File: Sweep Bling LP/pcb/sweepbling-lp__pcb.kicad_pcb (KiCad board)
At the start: 2 copper layers, 216.9 x 86.9 mm, 93 parts, among them J1 Conn_01x05, J1_r1 Conn_01x05, SW1 SW_Push, SW10 SW_Push, SW10_r1 SW_Push, SW11 SW_Push, SW11_r1 SW_Push, SW12 SW_Push, SW12_r1 SW_Push, SW13 SW_Push, SW13_r1 SW_Push, SW14 SW_Push, SW14_r1 SW_Push, SW15 SW_Push, SW15_r1 SW_Push, SW16 SW_Push, SW16_r1 SW_Push, SW17 SW_Push, SW17_r1 SW_Push, SW1_r1 SW_Push, SW2 SW_Push, SW2_r1 SW_Push, SW3 SW_Push, SW3_r1 SW_Push, SW4 SW_Push, SW4_r1 SW_Push, SW5 SW_Push, SW5_r1 SW_Push, SW6 SW_Push, SW6_r1 SW_Push, SW7 SW_Push, SW7_r1 SW_Push, SW8 SW_Push, SW8_r1 SW_Push, SW9 SW_Push, SW9_r1 SW_Push, U1 ProMicro-kbd, U2 ProMicro-kbd

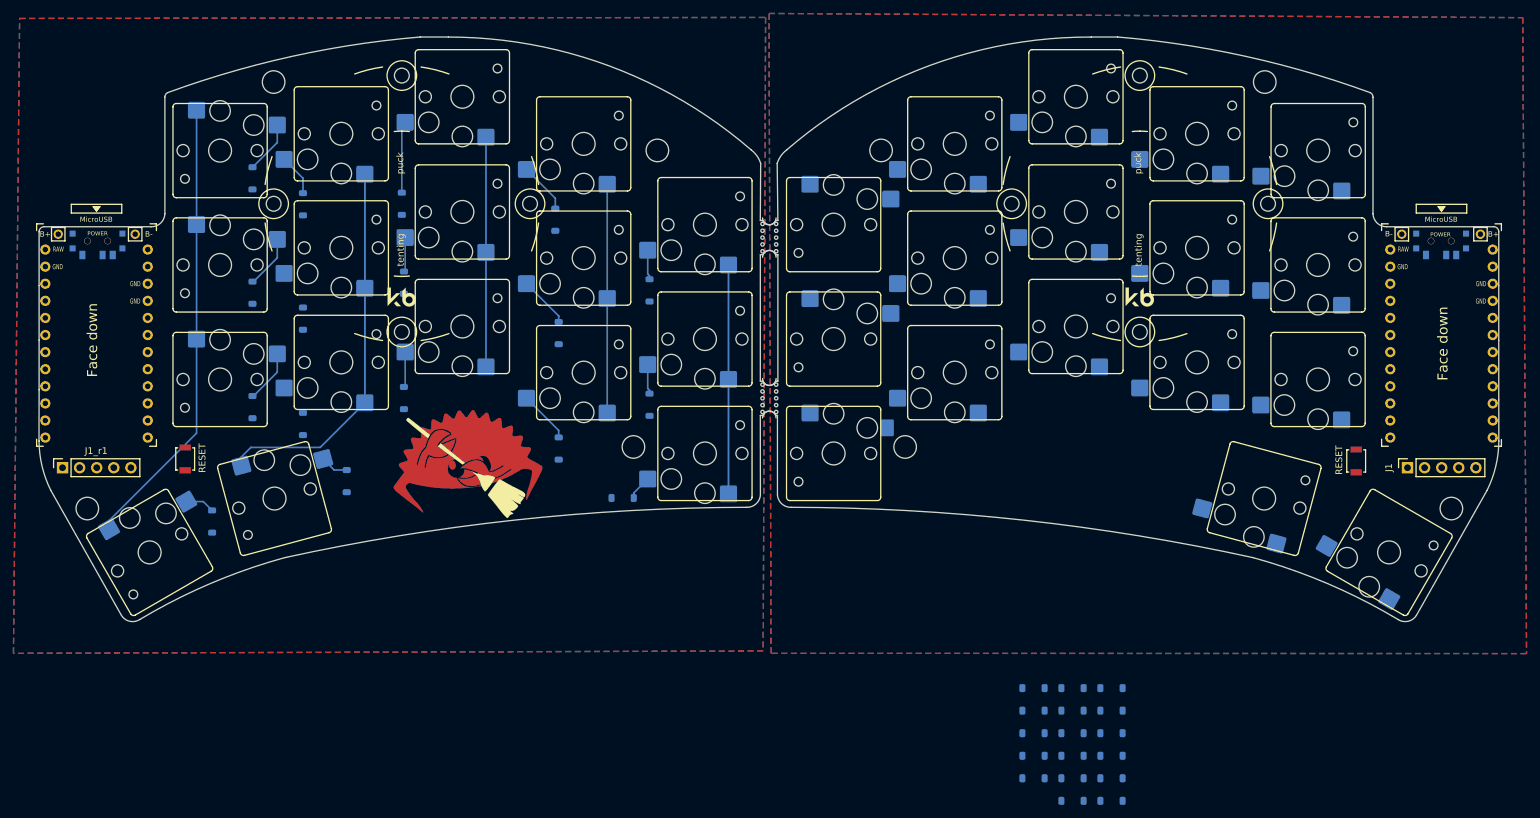
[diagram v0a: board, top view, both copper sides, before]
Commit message: traces addition
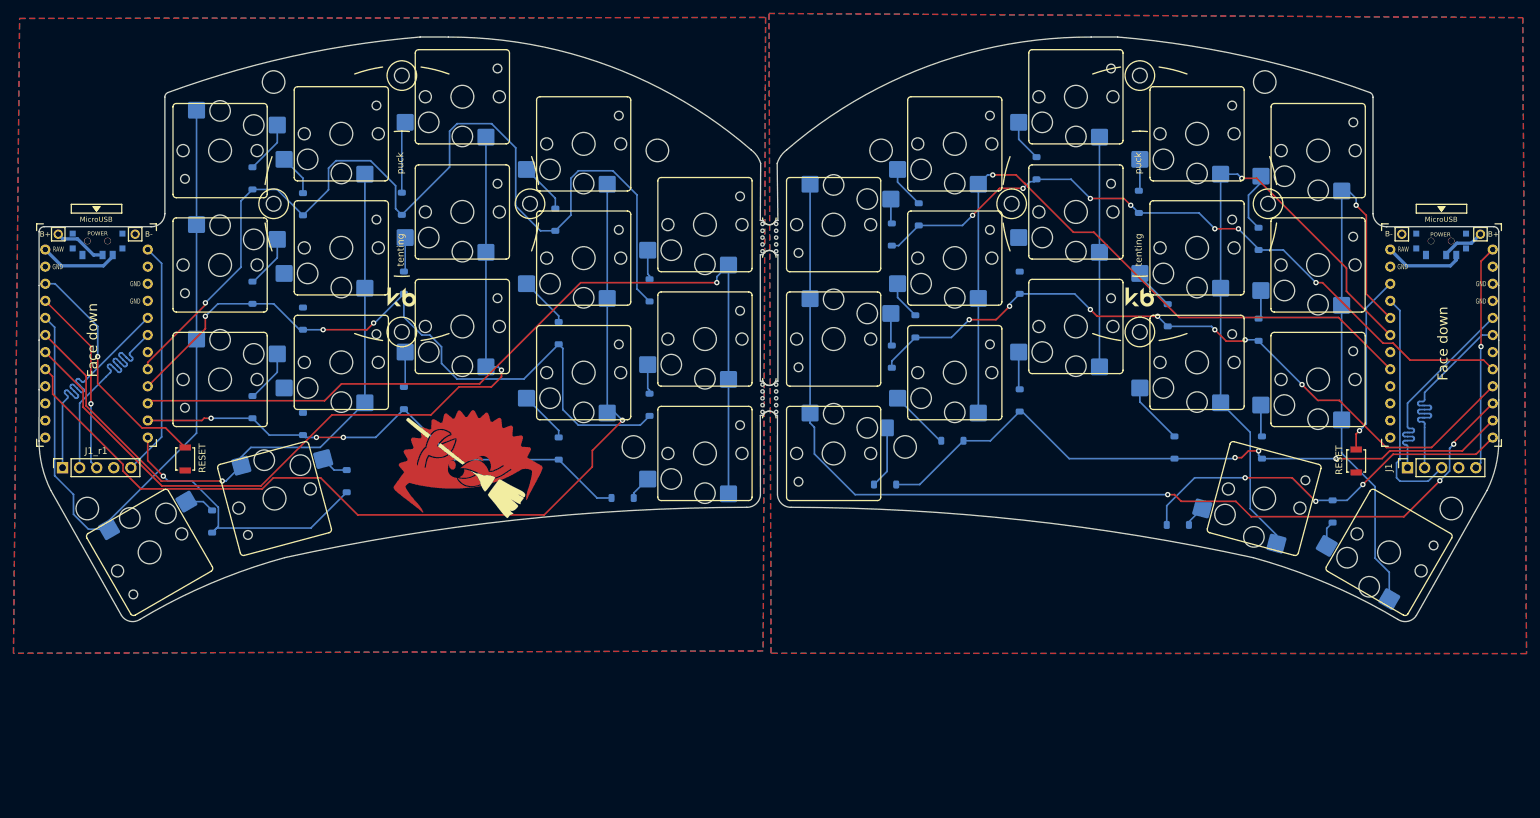
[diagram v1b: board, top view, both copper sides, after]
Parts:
- moved D20 84.7 mm to (170.0, 41.0), turned to 90 degrees
- moved D22 83.1 mm to (203.0, 51.5), turned to 90 degrees
- moved D21 82.4 mm to (185.2, 46.0), turned to 90 degrees
- moved D19 79.1 mm to (152.5, 47.9), turned to 90 degrees
- moved D18 74.9 mm to (148.5, 50.9), turned to 90 degrees
- moved D23 73.6 mm to (148.5, 69.0), turned to 90 degrees
- moved D27 69.1 mm to (203.0, 65.0), turned to 90 degrees
- moved D25 64.1 mm to (167.5, 58.0), turned to 90 degrees
- moved D26 63.7 mm to (189.5, 62.9), turned to 90 degrees
- moved D34 59.6 mm to (214.0, 92.0), turned to -90 degrees
- moved D24 58.6 mm to (152.0, 64.5), turned to 90 degrees
- moved D29 56.4 mm to (157.5, 81.5)
- moved D32 54.4 mm to (203.5, 82.5), turned to 90 degrees
- moved D28 51.8 mm to (147.5, 88.0)
- moved D31 44.4 mm to (190.5, 82.5), turned to 90 degrees
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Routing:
- net Switch1: track 0.00 -> 154.1 mm, vias 0 -> 3
- net Switch14_r: track 0.00 -> 147.9 mm, vias 0 -> 1
- net Switch2_r: track 34.0 -> 142.1 mm, vias 0 -> 1
- net Switch15: track 0.00 -> 108.0 mm, vias 0 -> 7
- net Switch2: track 0.00 -> 107.8 mm, vias 0 -> 1
- net Switch15_r: track 0.00 -> 106.3 mm, vias 0 -> 3
- net Switch14: track 0.00 -> 105.1 mm, vias 0 -> 7
- net Switch16: track 0.00 -> 99.7 mm, vias 0 -> 3
- net Switch4: track 0.00 -> 95.5 mm, vias 0 -> 1
- net Switch1_r: track 34.0 -> 129.3 mm, vias 0 -> 1
- net Switch3_r: track 34.1 -> 121.9 mm, vias 0 -> 1
- net Switch5: track 0.00 -> 86.0 mm, vias 0 -> 1
- net Switch16_r: track 0.00 -> 77.4 mm, vias 0 -> 3
- net Switch17: track 0.00 -> 58.4 mm, vias 0 -> 3
- net Switch17_r: track 0.00 -> 43.4 mm, vias 0 -> 1
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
